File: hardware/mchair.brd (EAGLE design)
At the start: 25.6 x 53.5 mm, 120 parts, among them J1 UX60-MB-5S8, J2 JTAG-MINI, U1 STM32F769NIH6, U2 S25FS256SAGNFI00, U3 LAN8742A, U4 USB3315C, U5 MIC5503-1.8YMT-TR, U6 MT48LC16M16A2F4, U7 MPM3620GQV-P, U8 NCP186AMX330TAG, X1 G83270021, X2 DSC6101JI2A-025.0000, X3 DSC6101JI2A-024.0000

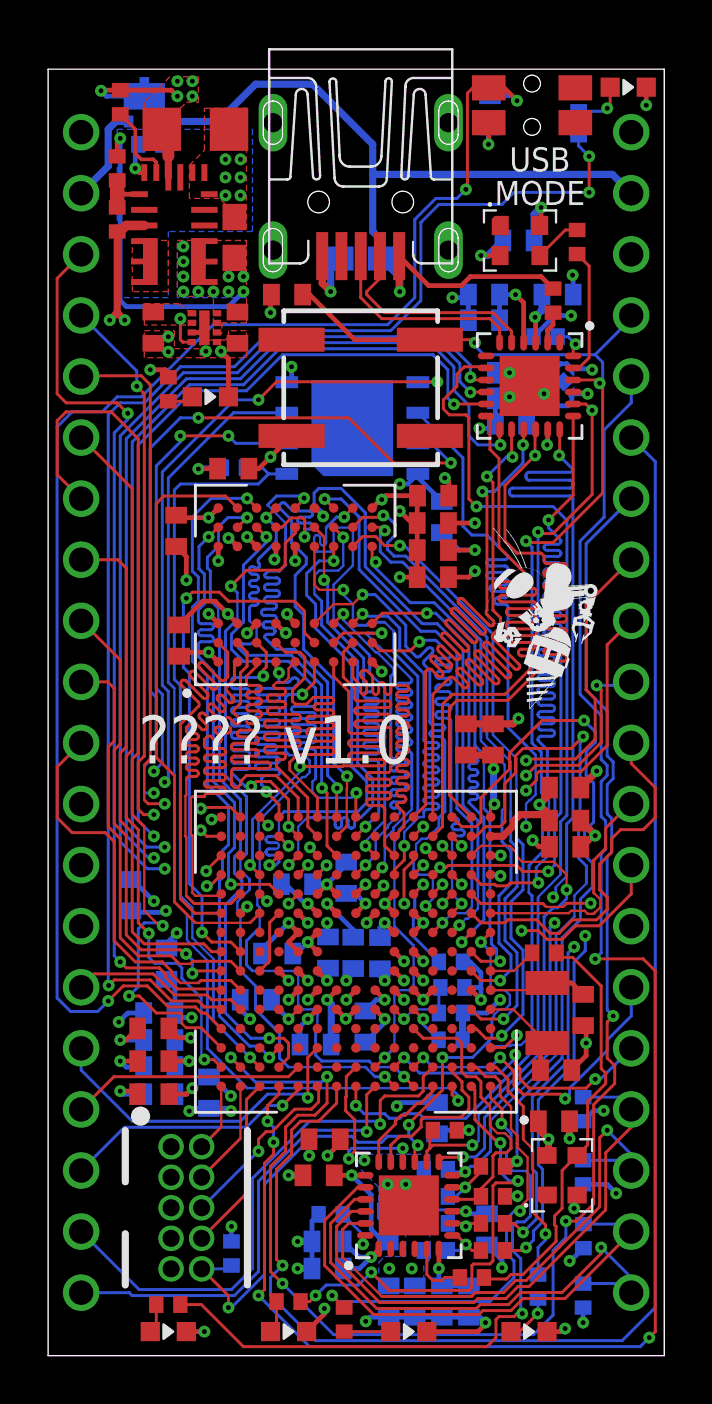
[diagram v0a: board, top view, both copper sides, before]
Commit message: Start 6 layer routing
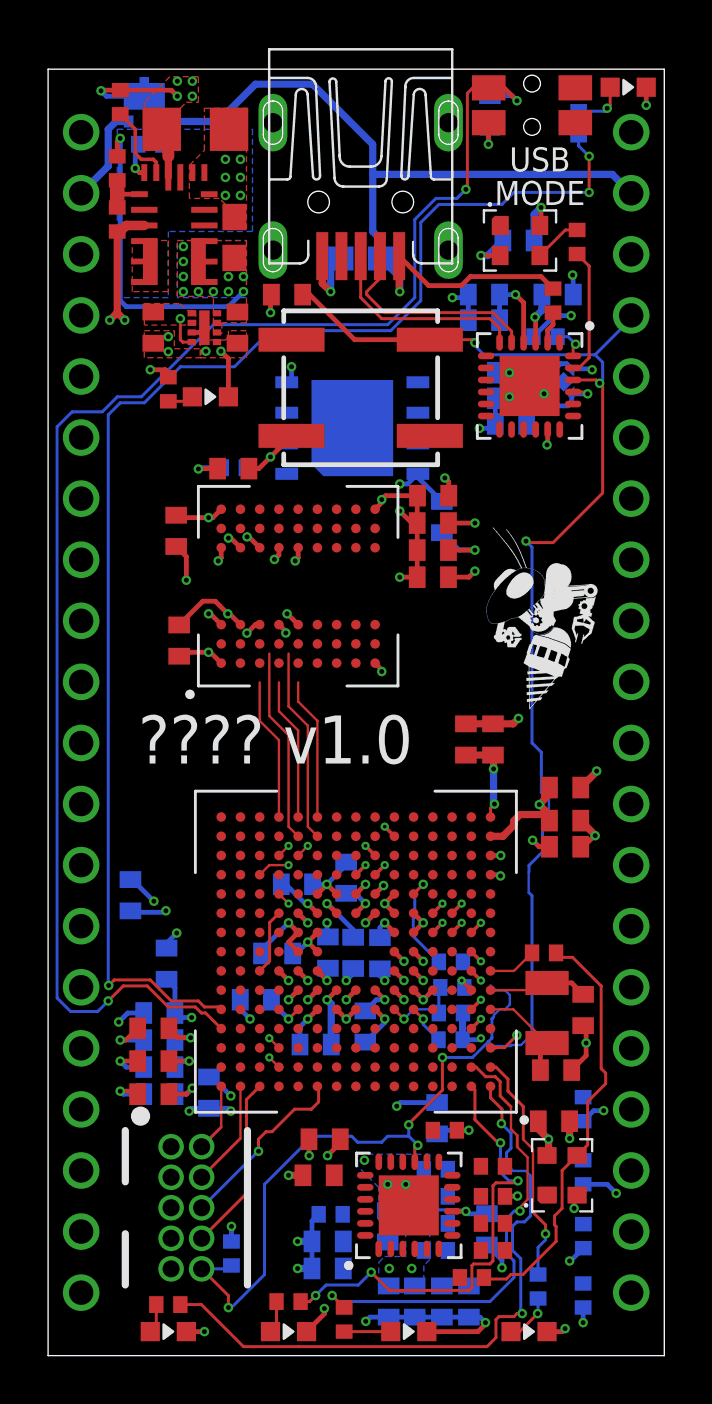
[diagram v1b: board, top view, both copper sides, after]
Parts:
- moved U6 0.13 mm to (10.4, 32.0)
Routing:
- net OUT-E1: track 70.5 -> 0.00 mm, vias 5 -> 0
- net OUT-E3: track 64.9 -> 0.00 mm, vias 5 -> 0
- net OUT-E2: track 64.4 -> 0.00 mm, vias 1 -> 0
- net OTG_HS-D7: track 44.4 -> 0.00 mm, vias 2 -> 0
- net OTG_HS-D3: track 44.2 -> 0.00 mm, vias 3 -> 0
- net QSPI-D2: track 42.6 -> 0.00 mm, vias 1 -> 0
- net OTG_HS-D6: track 42.5 -> 0.00 mm, vias 3 -> 0
- net OTG_HS-D5: track 42.0 -> 0.00 mm, vias 3 -> 0
- net OTG_HS-D4: track 39.7 -> 0.00 mm, vias 3 -> 0
- net QSPI-D3: track 39.6 -> 0.00 mm, vias 4 -> 0
- net OUT-B1: track 37.7 -> 0.00 mm, vias 2 -> 0
- net OUT-B5: track 37.4 -> 0.00 mm, vias 2 -> 0
- net QSPI-D0: track 35.1 -> 0.00 mm, vias 4 -> 0
- net OTG_HS-NXT: track 34.4 -> 0.00 mm, vias 3 -> 0
- net OTG_HS-STP: track 34.3 -> 0.00 mm, vias 3 -> 0
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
